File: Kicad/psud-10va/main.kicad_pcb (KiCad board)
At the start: 2 copper layers, 120 x 60 mm, 57 parts, among them K1 MAIN AC, K2 PSU1, K3 PSU2, X101 LOGO

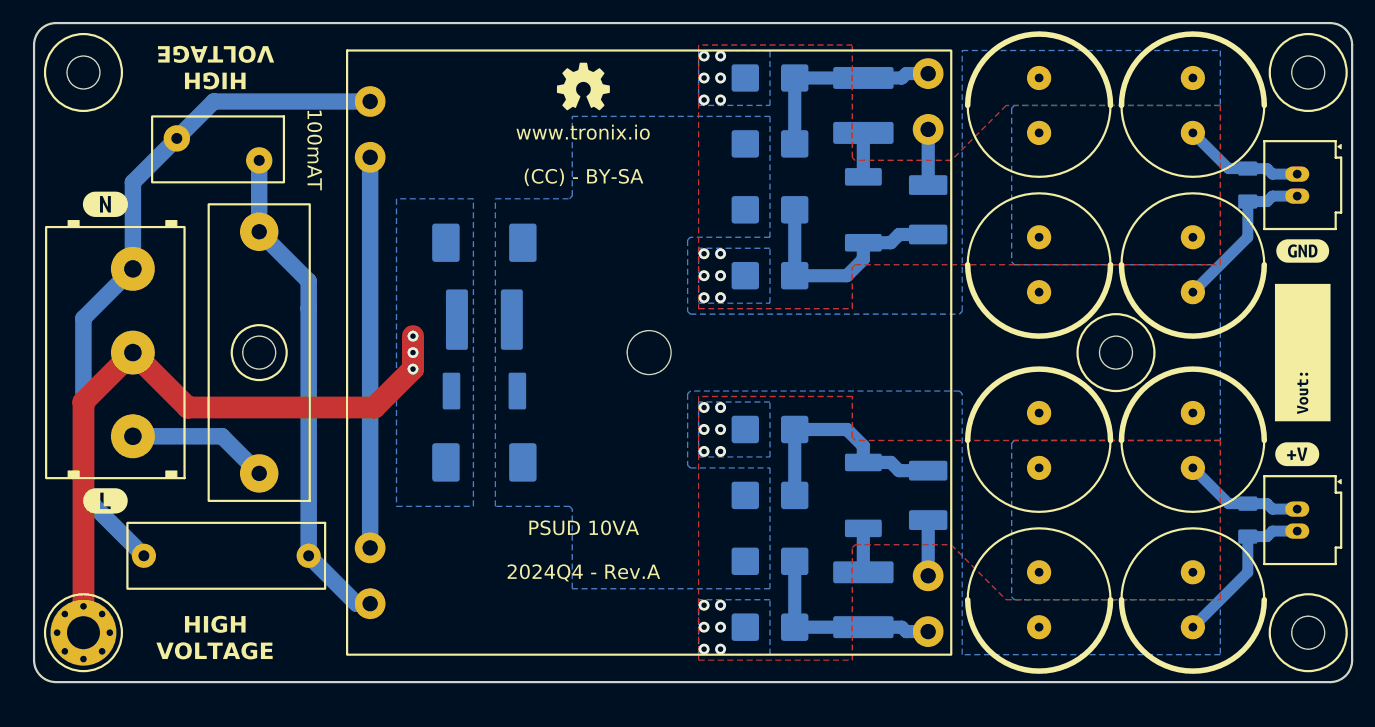
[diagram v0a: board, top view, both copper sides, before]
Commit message: Up
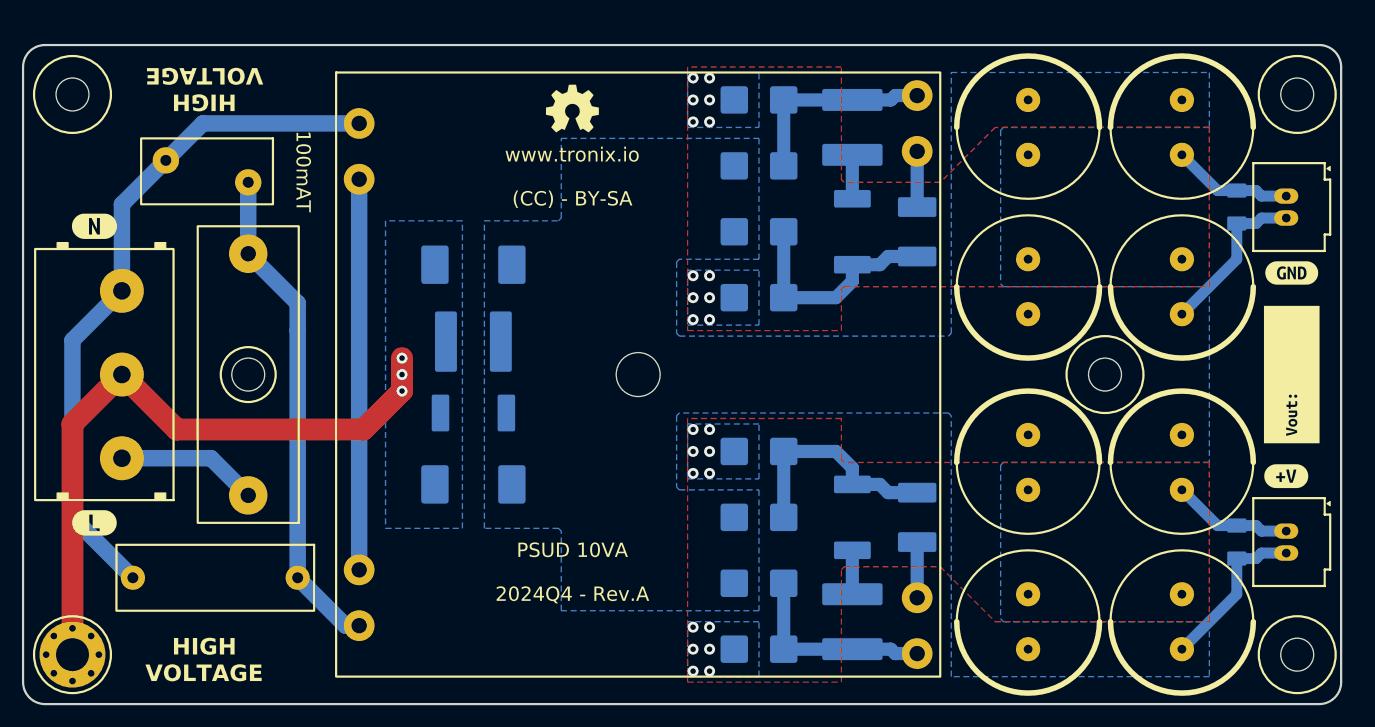
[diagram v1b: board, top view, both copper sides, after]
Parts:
- moved C1 2.24 mm to (102.5, 108.5)
- moved C10 2.24 mm to (190.5, 82.0)
- moved C11 2.24 mm to (190.5, 98.0)
- moved C12 2.24 mm to (195.5, 74.8)
- moved C13 2.24 mm to (195.5, 105.2)
- moved C14 2.24 mm to (126.0, 87.0)
- moved C2 2.24 mm to (160.5, 67.5)
- moved C3 2.24 mm to (160.5, 112.5)
- moved C4 2.24 mm to (176.5, 67.5)
- moved C5 2.24 mm to (176.5, 112.5)
- moved C6 2.24 mm to (176.5, 82.0)
- moved C7 2.24 mm to (176.5, 98.0)
- moved C8 2.24 mm to (190.5, 67.5)
- moved C9 2.24 mm to (190.5, 112.5)
- moved D1 2.24 mm to (152.0, 83.0)
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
